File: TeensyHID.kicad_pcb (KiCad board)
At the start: 2 copper layers, 35.6 x 26.5 mm, 11 parts, among them P1/SCL1 Conn_01x02, P2/SDA1 Conn_01x02, P3/SCL0 Conn_01x02, P4/SDA0 Conn_01x02, SW1 Rotary_Encoder_Switch, SW1POS2 Rotary_Encoder_Switch, SW2 Rotary_Encoder_Switch, U1 Teensy-LC

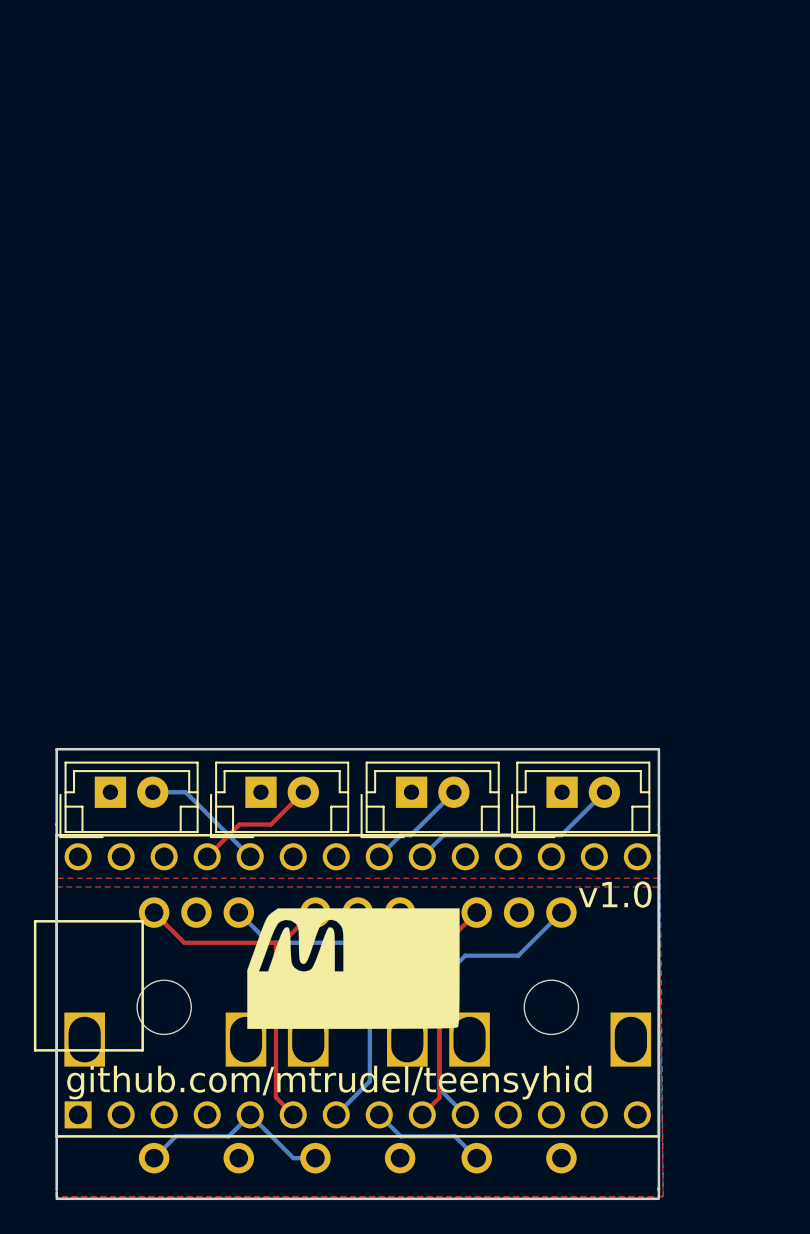
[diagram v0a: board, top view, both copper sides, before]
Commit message: 1.1 build of TeensyHID
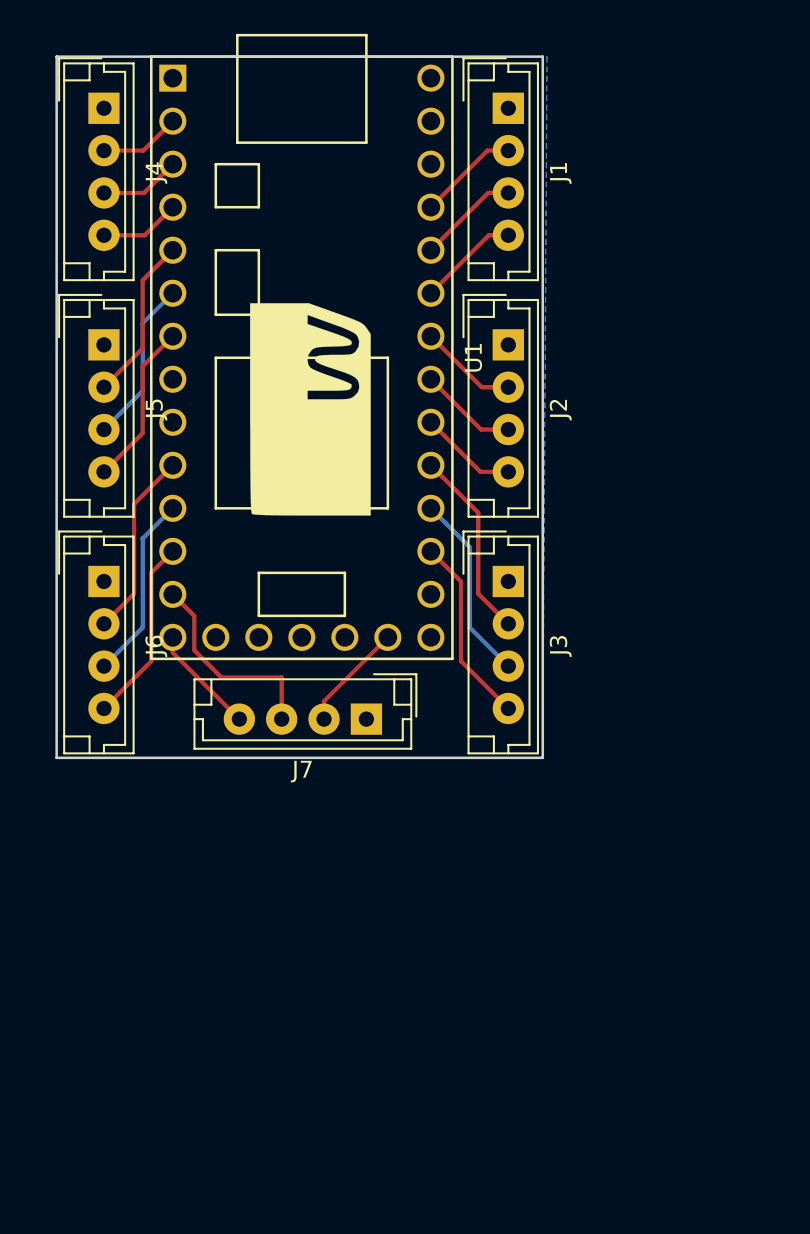
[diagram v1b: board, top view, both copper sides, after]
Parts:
- removed P1/SCL1, P2/SDA1, P3/SCL0, P4/SDA0: Conn_01x02, Connectors_JST:JST_EH_B02B-EH-A_02x2.50mm_Straight
- removed REF** (x2): MountingHole_3.2mm_M3, Mounting_Holes:MountingHole_3.2mm_M3
- removed SW1, SW1POS2, SW2: Rotary_Encoder_Switch, Local Copy:PEC11R-4xxx-Sxxxx
- added J1: Conn_01x04, Connectors_JST:JST_EH_B04B-EH-A_04x2.50mm_Straight, F.Cu at (138.4, 54.9)
- added J2: Conn_01x04, Connectors_JST:JST_EH_B04B-EH-A_04x2.50mm_Straight, F.Cu at (138.4, 68.8)
- added J3: Conn_01x04, Connectors_JST:JST_EH_B04B-EH-A_04x2.50mm_Straight, F.Cu at (138.4, 82.8)
- added J4: Conn_01x04, Connectors_JST:JST_EH_B04B-EH-A_04x2.50mm_Straight, F.Cu at (114.6, 54.9)
- added J5: Conn_01x04, Connectors_JST:JST_EH_B04B-EH-A_04x2.50mm_Straight, F.Cu at (114.6, 68.8)
- added J6: Conn_01x04, Connectors_JST:JST_EH_B04B-EH-A_04x2.50mm_Straight, F.Cu at (114.6, 82.8)
- added J7: Conn_01x04, Connectors_JST:JST_EH_B04B-EH-A_04x2.50mm_Straight, F.Cu at (130.0, 90.9)
- U1: footprint teensy:Teensy30_31_32_LC -> Teensy:Teensy30_31_32_LC
- moved U1 37.2 mm to (126.2, 69.6), turned to 270 degrees
- moved G*** 33.1 mm to (126.7, 72.6), turned to 270 degrees
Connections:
- U1 pad 11: (no net) -> Net-(J6-Pad3)
- U1 pad 12: (no net) -> Net-(J6-Pad4)
- U1 pad 13: (no net) -> Net-(J7-Pad3)
- U1 pad 14: (no net) -> Net-(J7-Pad4)
- U1 pad 2: (no net) -> Net-(J4-Pad2)
- U1 pad 22: (no net) -> Net-(J3-Pad4)
- U1 pad 23: (no net) -> Net-(J3-Pad3)
- U1 pad 24: (no net) -> Net-(J3-Pad2)
- U1 pad 27: (no net) -> Net-(J2-Pad2)
- U1 pad 28: (no net) -> Net-(J1-Pad4)
- U1 pad 3: (no net) -> Net-(J4-Pad3)
- U1 pad 32: Net-(P1/SCL1-Pad1) -> GND
- U1 pad 4: (no net) -> Net-(J4-Pad4)
- U1 pad 8: Net-(SW2-Pad5) -> (no net)
- U1 pad 9: Net-(SW2-Pad3) -> (no net)
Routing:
- net Net-(SW2-Pad3): track 13.3 -> 0.00 mm
- net Net-(J5-Pad4): track 22.0 -> 9.69 mm
- net Net-(J7-Pad3): track 0.00 -> 12.1 mm
- net Net-(J5-Pad3): track 21.6 -> 9.73 mm
- net Net-(J3-Pad2): track 0.00 -> 11.3 mm
- net Net-(J3-Pad3): track 0.00 -> 11.2 mm
- net Net-(J3-Pad4): track 0.00 -> 11.2 mm
- net Net-(J6-Pad3): track 0.00 -> 11.0 mm
- net Net-(J6-Pad4): track 0.00 -> 11.0 mm
- net Net-(SW2-Pad5): track 6.81 -> 0.00 mm
- net Net-(J2-Pad4): track 12.3 -> 5.78 mm
- net Net-(J7-Pad4): track 0.00 -> 6.45 mm
- net Net-(J7-Pad2): track 0.00 -> 6.39 mm
- net Net-(J6-Pad2): track 17.4 -> 11.0 mm
- net Net-(J1-Pad4): track 0.00 -> 5.99 mm
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- removed copper zone on F.Cu, net Net-(P1/SCL1-Pad1)
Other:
- board size 35.6 x 26.5 mm -> 28.7 x 41.4 mm
- board text removed: "github.com/mtrudel/teensyhid"
- board text removed: "v1.0"
